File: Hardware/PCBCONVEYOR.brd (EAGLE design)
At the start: 68 x 54 mm, 8 parts, among them J1 SPI-LCD, J11 IO, J2 I2CBR, J3 M06-PLAIN, J4 SPI-LCD, J5 I2CBR, J6 M12-PLAIN, J7 M12-PLAIN

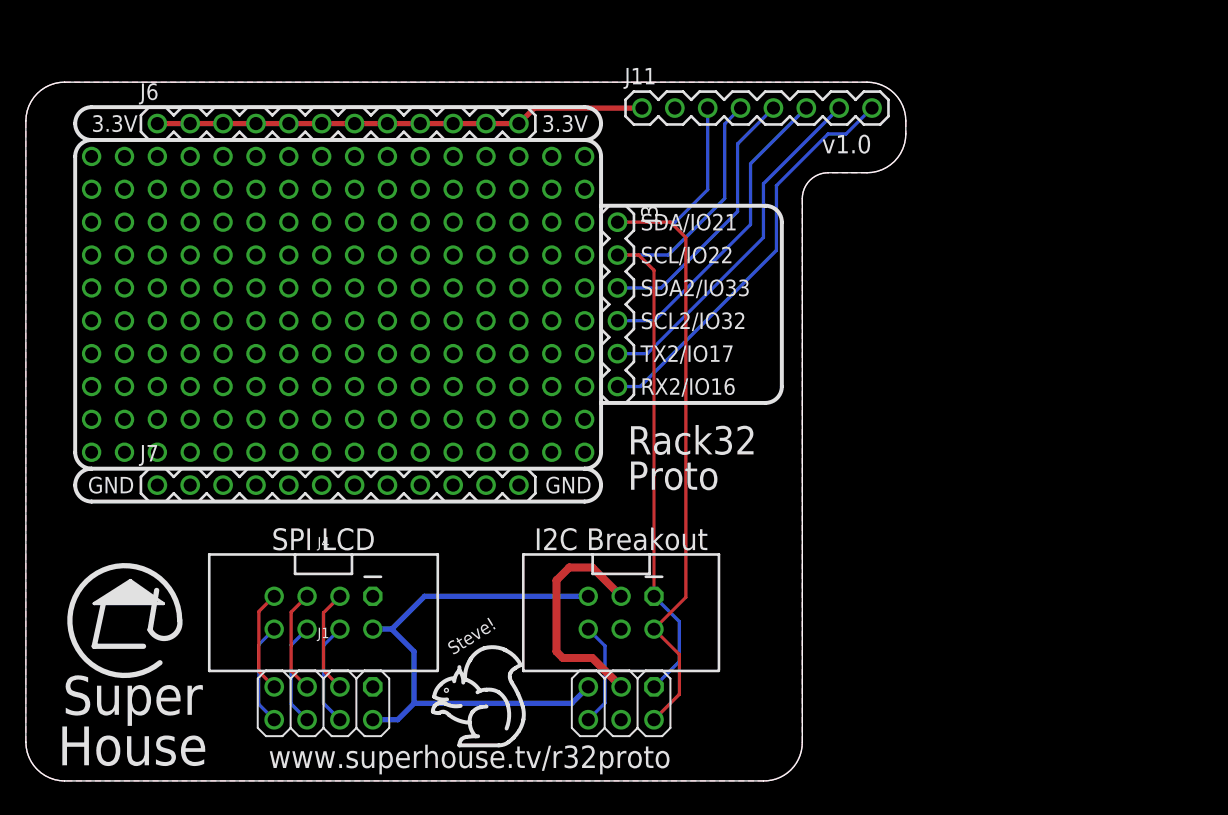
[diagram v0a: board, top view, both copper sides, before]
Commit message: v1.0 release.
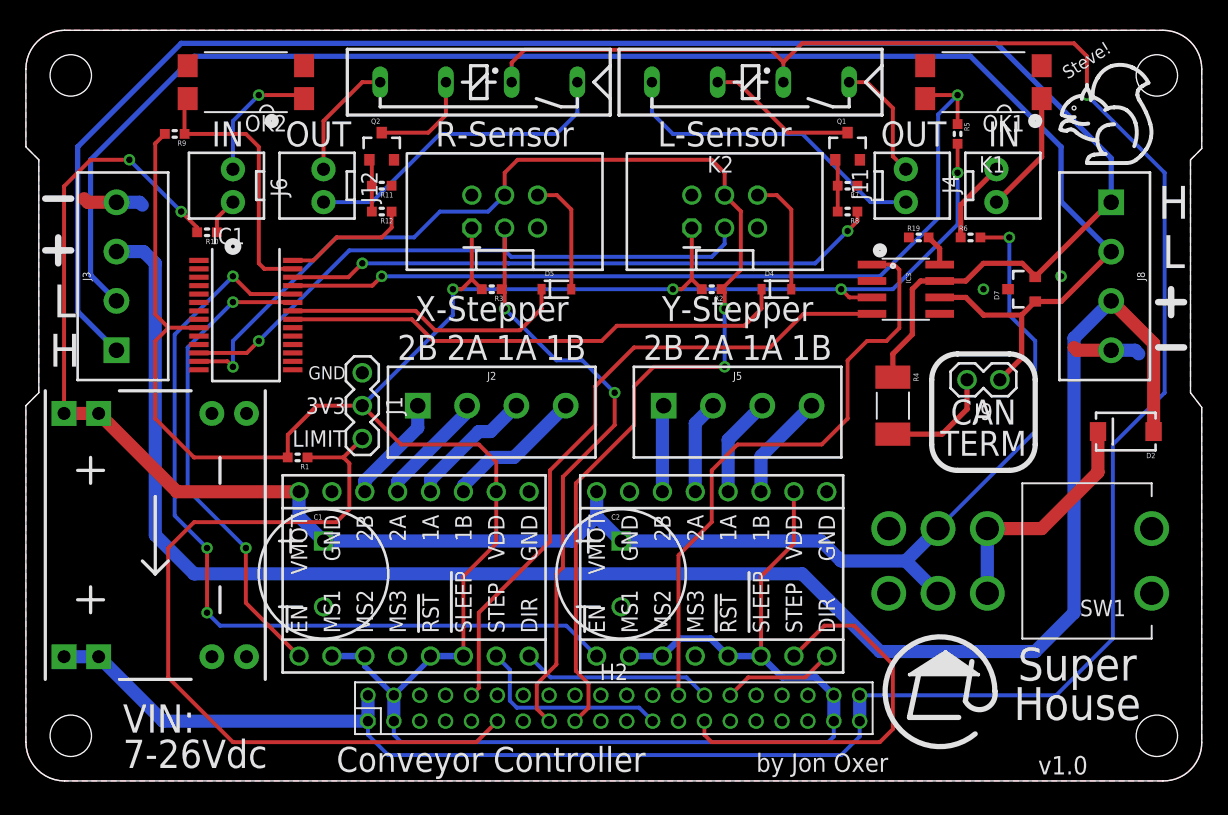
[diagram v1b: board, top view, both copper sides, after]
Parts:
- added C1, C2: 220uF, SuperHouse-Capacitors:CPOL-RADIAL-220UF-50V
- added D2: SS56, SuperHouse-Diodes:SMA-DIODE
- added D4, D5: (no value), SuperHouse-Diodes:SOD-323
- added D7: TVSDUAL-T24CAN, SuperHouse-Diodes:SOT23-3
- added H2: M02X20-2.00-P-BELOW, SuperHouse-Connectors:2X20-2.00-P-BELOW
- added IC1: MCP23017SS, SuperHouse-ICs:SSOP28
- added IC3: TCAN332DR, SuperHouse-ICs:SO08
- added J10: SENSOR_R, SuperHouse-Connectors:2X3-2.54-SHROUDED
- added J12: Right Output, SuperHouse-Connectors:1X02-KF2510
- added J8: CAN_BUS, SuperHouse-Connectors:SCREWTERMINAL-3.81MM-VERT-4
- added J9: CAN_TERM, SuperHouse-Connectors:1X02-P-JUMP-Y
- added K1, K2: REED-SIL, SuperHouse-Relays:REED
- added MOD1, MOD2: STEPSTICK, SuperHouse-MotorDrivers:STEPSTICK
- added OK1, OK2: LTV816-SMT, SuperHouse-LEDs:SMD4
- added Q1, Q2: 2N7002, SuperHouse-Transistors:SOT23-3
- added R1, R11, R19, R5, R7, R9: 10K, SuperHouse-Resistors:R0603
- added R10, R6: 560R, SuperHouse-Resistors:R0603
- added R12, R8: 1K, SuperHouse-Resistors:R0603
- added R2, R3: 4K7, SuperHouse-Resistors:R0603
- added R4: 120R, SuperHouse-Resistors:R2010
- added SW1: Power, SuperHouse-Switches:7201SD9AV2BE
- added VR1: DC5V3A-PTH, SuperHouse-Regulators:DC5V3A-PTH
- J1: value SPI-LCD -> Limit Sensor; device SuperHouse-Connectors:2X04-S-BELOW -> SuperHouse-Connectors:1X03-P
- J11: value IO -> Left Output; device SuperHouse-Connectors:1X08-P-BELOW -> SuperHouse-Connectors:1X02-KF2510
- J2: value I2CBR -> (none); device SuperHouse-Connectors:2X03-S-BELOW -> SuperHouse-Connectors:SCREWTERMINAL-3.81MM-VERT-4
- J3: value M06-PLAIN -> CAN_BUS; device SuperHouse-Connectors:1X06 -> SuperHouse-Connectors:SCREWTERMINAL-3.81MM-VERT-4
- J4: value SPI-LCD -> Left Input; device SuperHouse-Connectors:2X04-2.54-SHROUDED -> SuperHouse-Connectors:1X02-KF2510
- J5: value I2CBR -> (none); device SuperHouse-Connectors:2X3-2.54-SHROUDED -> SuperHouse-Connectors:SCREWTERMINAL-3.81MM-VERT-4
- J6: value M12-PLAIN -> Right Input; device SuperHouse-Connectors:1X12 -> SuperHouse-Connectors:1X02-KF2510
- J7: value M12-PLAIN -> SENSOR_L; device SuperHouse-Connectors:1X12 -> SuperHouse-Connectors:2X3-2.54-SHROUDED
- moved J4 61.6 mm to (75.0, 46.0), turned to 90 degrees
- moved J7 48.7 mm to (54.0, 44.0)
- moved J3 38.8 mm to (7.00, 39.0), turned to 90 degrees
- moved J2 25.1 mm to (36.0, 29.0), turned to 0 degrees
- moved J1 23.2 mm to (26.0, 29.0), turned to 270 degrees
- moved J5 18.4 mm to (55.0, 29.0), turned to 0 degrees
- moved J11 13.0 mm to (68.0, 46.0), turned to 90 degrees
- moved J6 7.56 mm to (16.0, 46.0), turned to 270 degrees
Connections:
- removed net !RESET: J2.6, J5.6
- removed net 12V: J2.3, J5.3
- removed net IO14_TFT_BLK: J1.7, J4.7
- removed net IO16_RX2: J11.8, J3.6
- removed net IO17_TX2: J11.7, J3.5
- removed net IO18_SCLK: J1.3, J4.3
- removed net IO21_SDA: J11.3, J2.2, J3.1, J5.2
- removed net IO22_SCL: J11.4, J2.1, J3.2, J5.1
- removed net IO23_COPI: J1.4, J4.4
- removed net IO25_TFT_CS: J1.8, J4.8
- removed net IO2_TFT_DC: J1.6, J4.6
- removed net IO32_SCL2: J11.6, J3.4
- removed net IO33_SDA2: J11.5, J3.3
- removed net IO4_TFT_RST: J1.5, J4.5
- new net 5V: H2.1, H2.2, H2.39, H2.40, K1.3, K2.3, VR1.3A, VR1.3B
- new net CAN_H1: D7.2, IC3.7, J3.1, J8.1, R4.1
- new net CAN_L1: D7.1, IC3.6, J3.2, J8.2, J9.1
- new net CAN_VIN: D2.A, J3.3, J8.3
- new net ESP_EN: H2.18
- new net GPA0_XSHUT_L: D4.1, IC1.21
- new net GPA1_XSHUT_R: D5.1, IC1.22
- new net GPA2_!X_ENABLE: IC1.23, MOD2.1
- new net GPA3_!Y_ENABLE: IC1.24, MOD1.1
- new net GPA4_LEFT_IN: IC1.25, OK1.4, R5.1
- new net GPA5_LEFT_OUT: IC1.26, R8.1
- new net GPA6_RIGHT_IN: IC1.27, OK2.4, R9.1
- new net GPA7_RIGHT_OUT: IC1.28, R12.1
- new net GPB0: IC1.1
- new net GPB1: IC1.2
- new net GPB2: IC1.3
- new net GPB3: IC1.4
- new net GPB4: IC1.5
- new net GPB5: IC1.6
- new net GPB6: IC1.7
- new net GPB7: IC1.8
- new net IO0: H2.24
- new net IO12_X_STEP: H2.23, MOD2.7
- new net IO13_LCD_COPI: H2.16
- new net IO14_LCD_CLK: H2.25
- new net IO15_LCD_CS: H2.14
- new net IO18_I2C_SDA: H2.17, IC1.13, J10.4, J7.4, R2.1
- new net IO19_I2C_SCL: H2.15, IC1.12, J10.3, J7.3, R3.1
- new net IO2: H2.12
- new net IO21_LCD_RS: H2.19
- new net IO22_LCD_RST: H2.20
- new net IO23_LCD_BL: H2.22
- new net IO25_X_DIR: H2.28, MOD2.8
- new net IO26_Y_DIR: H2.30, MOD1.8
- new net IO27_Y_STEP: H2.27, MOD1.7
- new net IO32: H2.29
- new net IO33: H2.31
- new net IO34: H2.13
- new net IO35: H2.32
- new net IO36: H2.9
- new net IO39_LIMIT: H2.11, J1.3, R1.1
- new net IO4_CAN_RX: H2.10, IC3.4
- new net IO5_CAN_TX: H2.26, IC3.1
- new net N$1: J2.1, MOD2.14
- new net N$2: IC3.8, R19.2
- new net N$20: J9.2, R4.2
- new net N$21: J2.2, MOD2.13
- new net N$22: D5.2, J10.6
- new net N$24: J4.1, OK1.1
- new net N$25: J5.1, MOD1.14
- new net N$26: J4.2, R6.1
- new net N$27: D4.2, J7.6
- new net N$28: K1.5, Q1.3
- new net N$29: J5.2, MOD1.13
- new net N$3: IC1.18
- new net N$30: J5.3, MOD1.12
- new net N$31: J11.2, K1.1
- new net N$32: Q1.1, R7.2, R8.2
- new net N$34: J11.1, K1.7
- new net N$35: J5.4, MOD1.11
- new net N$36: Q2.1, R11.2, R12.2
- new net N$38: K2.5, Q2.3
- new net N$40: J12.2, K2.1
- new net N$41: J12.1, K2.7
- new net N$42: J6.1, OK2.1
- new net N$43: J6.2, R10.1
- new net N$44: J2.3, MOD2.12
- new net N$45: J2.4, MOD2.11
- new net TXD: H2.21
- new net VIN: D2.C, SW1.1, SW1.6
- new net VSWITCHED: C1.1, C2.1, MOD1.16, MOD2.16, R10.2, R6.2, SW1.2, SW1.5, VR1.2A, VR1.2B
- net 3.3V: now also H2.3, H2.37, H2.38, H2.4, IC1.9, IC3.3, J10.1, J7.1, MOD1.10, MOD1.2, MOD1.3, MOD1.5, MOD1.6, MOD2.10, MOD2.2, MOD2.3, MOD2.5, MOD2.6, R1.2, R2.2, R3.2, R5.2, R9.2; no longer J11.1, J2.5, J4.2, J5.5, J6.1, J6.10, J6.11, J6.12, J6.2, J6.3, J6.4, J6.5, J6.6, J6.7, J6.8, J6.9
- net GND: now also C1.2, C2.2, D7.3, H2.33, H2.34, H2.35, H2.36, H2.5, H2.6, H2.7, H2.8, IC1.10, IC1.15, IC1.16, IC1.17, IC3.2, J10.2, J3.4, J8.4, MOD1.15, MOD1.4, MOD1.9, MOD2.15, MOD2.4, MOD2.9, OK1.2, OK1.3, OK2.2, OK2.3, Q1.2, Q2.2, R11.1, R19.1, R7.1, VR1.1A, VR1.1B, VR1.4A, VR1.4B; no longer J11.2, J2.4, J4.1, J5.4, J7.1, J7.10, J7.11, J7.12, J7.3, J7.4, J7.5, J7.6, J7.7, J7.8, J7.9
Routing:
- net 5V: track 0.00 -> 190.9 mm, vias 0 -> 1
- net 3.3V: track 79.8 -> 235.0 mm, vias 0 -> 4
- net VSWITCHED: track 0.00 -> 141.3 mm, vias 0 -> 3
- net CAN_VIN: track 0.00 -> 137.1 mm
- net CAN_H1: track 0.00 -> 133.7 mm
- net CAN_L1: track 0.00 -> 124.2 mm
- net IO18_I2C_SDA: track 0.00 -> 102.5 mm, vias 0 -> 3
- net IO19_I2C_SCL: track 0.00 -> 93.4 mm, vias 0 -> 3
- net GPA4_LEFT_IN: track 0.00 -> 67.0 mm, vias 0 -> 2
- net GPA3_!Y_ENABLE: track 0.00 -> 65.6 mm, vias 0 -> 3
- net IO39_LIMIT: track 0.00 -> 62.5 mm
- net IO21_SDA: track 60.0 -> 0.00 mm
- net IO22_SCL: track 54.7 -> 0.00 mm
- net IO4_CAN_RX: track 0.00 -> 51.5 mm
- net IO5_CAN_TX: track 0.00 -> 46.9 mm
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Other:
- board size 68 x 54 mm -> 90.9 x 58 mm
- board text added: "!INT"
- board text added: "!XSHUT"
- board text added: "1A"
- board text added: "1B"
- board text added: "2A"
- board text added: "2B"
- board text added: "3V3"
- board text added: "CAN TERM"
- board text added: "CAN_H"
- board text added: "CAN_L"
- board text added: "Conveyor Controller"
- board text added: "H"
- board text added: "IN"
- board text added: "L"
- board text added: "L-Sensor"
- board text added: "LIMIT"
- board text added: "OUT"
- board text added: "R-Sensor"
- board text added: "SCL"
- board text added: "SDA"
- board text added: "V+"
- board text added: "VIN+"
- board text added: "VIN: 7-26Vdc"
- board text added: "X-Stepper"
- board text added: "Y-Stepper"
- board text added: "by Jon Oxer"
- board text added: "www.superhouse.tv/conveyor"
- board text removed: "3.3V"
- board text removed: "I2C Breakout"
- board text removed: "RX2/IO16"
- board text removed: "Rack32 Proto"
- board text removed: "SCL/IO22"
- board text removed: "SCL2/IO32"
- board text removed: "SDA/IO21"
- board text removed: "SDA2/IO33"
- board text removed: "SPI LCD"
- board text removed: "TX2/IO17"
- board text removed: "www.superhouse.tv/r32proto"
